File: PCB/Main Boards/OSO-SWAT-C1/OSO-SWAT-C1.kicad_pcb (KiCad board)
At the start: 4 copper layers, 24.4 x 24.4 mm, 40 parts, among them J2 FH19C-9S-0.5SH_10_, Q1 Q_Photo_NPN, Q2 Q_NMOS_GSD, U1 ATSAML22J18A-MUT, U2 MIC5365-3.3YC5-TR, X1 Crystal

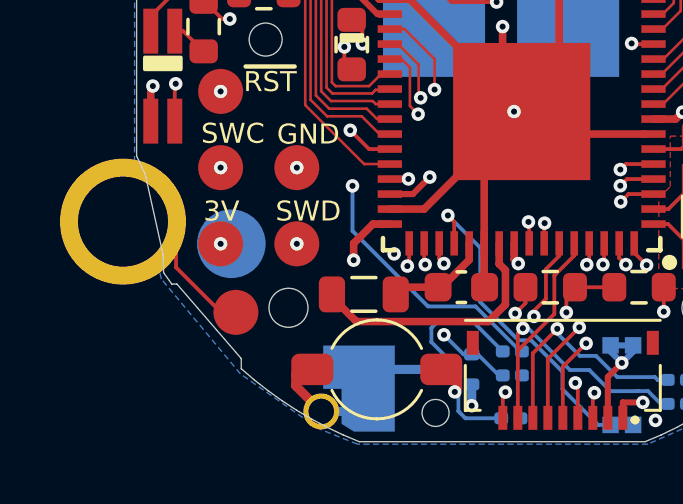
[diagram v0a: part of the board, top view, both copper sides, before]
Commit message: testjigulate, not routed
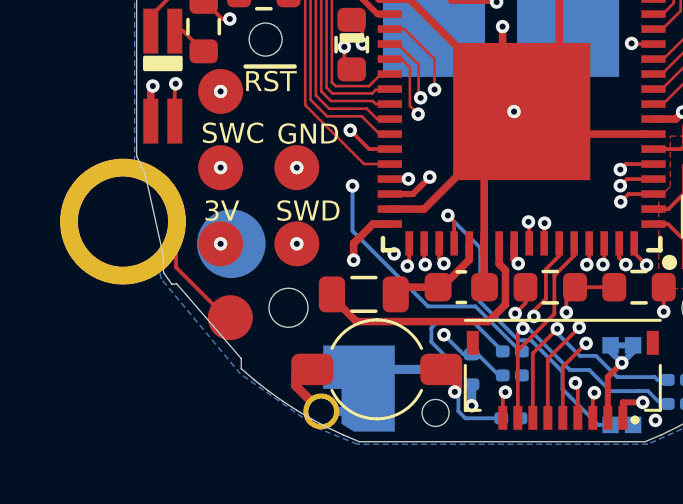
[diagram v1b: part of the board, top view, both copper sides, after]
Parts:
- moved TP9 0.26 mm to (3.10, 20.3)
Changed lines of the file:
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@@
 	(footprint "OSO-SWAT-A1-05:MICROBUILDER_TESTPOINT_ROUND_1.5MM"
 		(layer "F.Cu")
-		(at 3.285479 20.098521 180)
+		(at 3.1 20.275 180)
 		(property "Reference" "TP9"
 			(at 1.143 0.127 0)
@@
 	)
 	(segment
+		(start 1.29 18.103042)
+		(end 1.29 18.6)
+		(width 0.127)
+		(layer "F.Cu")
+		(net "/SWDIO_MODE")
+	)
+	(segment
+		(start 0.710408 16.80991)
+		(end 0.914679 17.727721)
+		(width 0.127)
+		(layer "F.Cu")
+		(net "/SWDIO_MODE")
+	)
+	(segment
+		(start 2.788521 20.098521)
+		(end 3.285479 20.098521)
+		(width 0.127)
+		(layer "F.Cu")
+		(net "/SWDIO_MODE")
+	)
+	(segment
+		(start 1.29 18.6)
+		(end 2.788521 20.098521)
+		(width 0.127)
+		(layer "F.Cu")
+		(net "/SWDIO_MODE")
+	)
+	(segment
+		(start 13.560479 17.799821)
+		(end 13.560479 17.139521)
+		(width 0.127)
+		(layer "F.Cu")
+		(net "/SWDIO_MODE")
+	)
+	(segment
+		(start 0.914679 17.727721)
+		(end 1.29 18.103042)
+		(width 0.127)
+		(layer "F.Cu")
+		(net "/SWDIO_MODE")
+	)
+	(segment
+		(start 13.560479 17.139521)
+		(end 13.575479 17.124521)
+		(width 0.127)
+		(layer "F.Cu")
+		(net "/SWDIO_MODE")
+	)
+	(via
+		(at 13.575479 17.124521)
+		(size 0.45)
+		(drill 0.2)
+		(layers "F.Cu" "B.Cu")
+		(capping no)
+		(covering
+			(front no)
+			(back no)
+		)
+		(plugging
+			(front no)
+			(back no)
+		)
+		(filling no)
+		(net "/SWDIO_MODE")
+	)
+	(via
+		(at 5.31548 17.81452)
+		(size 0.45)
+		(drill 0.2)
+		(layers "F.Cu" "B.Cu")
+		(capping no)
+		(covering
+			(front no)
+			(back no)
+		)
+		(plugging
+			(front no)
+			(back no)
+		)
+		(filling no)
+		(net "/SWDIO_MODE")
+	)
+	(segment
+		(start 5.55 17.58)
+		(end 13.12 17.58)
+		(width 0.127)
+		(layer "In1.Cu")
+		(net "/SWDIO_MODE")
+	)
+	(segment
+		(start 5.31548 17.81452)
+		(end 5.55 17.58)
+		(width 0.127)
+		(layer "In1.Cu")
+		(net "/SWDIO_MODE")
+	)
+	(segment
+		(start 13.12 17.58)
+		(end 13.575479 17.124521)
+		(width 0.127)
+		(layer "In1.Cu")
+		(net "/SWDIO_MODE")
+	)
+	(segment
+		(start 4.313733 16.812773)
+		(end 5.31548 17.81452)
+		(width 0.127)
+		(layer "In2.Cu")
+		(net "/SWDIO_MODE")
+	)
+	(segment
+		(start 4.313733 16.812773)
+		(end 0.697544 16.812773)
+		(width 0.127)
+		(layer "In2.Cu")
+		(net "/SWDIO_MODE")
+	)
+	(segment
 		(start 23.517703 16.928149)
 		(end 22.194979 18.250873)
@@
 	)
 	(segment
-		(start 1.29 18.103042)
-		(end 1.29 18.6)
-		(width 0.127)
-		(layer "F.Cu")
-		(net "/SWDIO_MODE")
-	)
-	(segment
-		(start 0.710408 16.80991)
-		(end 0.914679 17.727721)
-		(width 0.127)
-		(layer "F.Cu")
-		(net "/SWDIO_MODE")
-	)
-	(segment
-		(start 2.788521 20.098521)
-		(end 3.285479 20.098521)
-		(width 0.127)
-		(layer "F.Cu")
-		(net "/SWDIO_MODE")
-	)
-	(segment
-		(start 1.29 18.6)
-		(end 2.788521 20.098521)
-		(width 0.127)
-		(layer "F.Cu")
-		(net "/SWDIO_MODE")
-	)
-	(segment
-		(start 13.560479 17.799821)
-		(end 13.560479 17.139521)
-		(width 0.127)
-		(layer "F.Cu")
-		(net "/SWDIO_MODE")
-	)
-	(segment
-		(start 0.914679 17.727721)
-		(end 1.29 18.103042)
-		(width 0.127)
-		(layer "F.Cu")
-		(net "/SWDIO_MODE")
-	)
-	(segment
-		(start 13.560479 17.139521)
-		(end 13.575479 17.124521)
-		(width 0.127)
-		(layer "F.Cu")
-		(net "/SWDIO_MODE")
-	)
-	(via
-		(at 13.575479 17.124521)
-		(size 0.45)
-		(drill 0.2)
-		(layers "F.Cu" "B.Cu")
-		(capping no)
-		(covering
-			(front no)
-			(back no)
-		)
-		(plugging
-			(front no)
-			(back no)
-		)
-		(filling no)
-		(net "/SWDIO_MODE")
-	)
-	(via
-		(at 5.31548 17.81452)
-		(size 0.45)
-		(drill 0.2)
-		(layers "F.Cu" "B.Cu")
-		(capping no)
-		(covering
-			(front no)
-			(back no)
-		)
-		(plugging
-			(front no)
-			(back no)
-		)
-		(filling no)
-		(net "/SWDIO_MODE")
-	)
-	(segment
-		(start 5.55 17.58)
-		(end 13.12 17.58)
-		(width 0.127)
-		(layer "In1.Cu")
-		(net "/SWDIO_MODE")
-	)
-	(segment
-		(start 5.31548 17.81452)
-		(end 5.55 17.58)
-		(width 0.127)
-		(layer "In1.Cu")
-		(net "/SWDIO_MODE")
-	)
-	(segment
-		(start 13.12 17.58)
-		(end 13.575479 17.124521)
-		(width 0.127)
-		(layer "In1.Cu")
-		(net "/SWDIO_MODE")
-	)
-	(segment
-		(start 4.313733 16.812773)
-		(end 5.31548 17.81452)
-		(width 0.127)
-		(layer "In2.Cu")
-		(net "/SWDIO_MODE")
-	)
-	(segment
-		(start 4.313733 16.812773)
-		(end 0.697544 16.812773)
-		(width 0.127)
-		(layer "In2.Cu")
-		(net "/SWDIO_MODE")
-	)
-	(segment
